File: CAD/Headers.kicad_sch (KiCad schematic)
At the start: 62 parts, among them J1 SWD, J10 OUT_0, J11 OUT_1, J12 OUT_2, J13 TEMP_0, J14 TEMP_1, J15 TEMP_2, J16 EXPANSION, J17 ESP_DB, J18 250-502/000-006, J19 A2543WV-5P, J2 A2543WV-2P, J20 IO_1, J21 IO_2, J22 A2543WV-2P, J23 CAN_1_OUT, J24 DRIVER_2, J25 DRIVER_1, J26 DRIVER_0, J28 SPI_DB, J3 OUT_6, J30 LASER/VFD, J31 IO_3, J33 A2543WV-4P, J34 A2543WV-4P, J35 DRIVER_3, J36 DRIVER_4, J37 DRIVER_5, J38 CAN_0_OUT, J39 PANELDUE_SD, J4 OUT_7, J41 TEMP_3, J42 DS_LED, J44 IO_7_ISO_OUT, J47 IO_8_ISO_OUT, J48 SBC, J49 A2543WV-2P, J5 OUT_8, J50 EXT_5V_IN, J51 IO_4, J53 IO_5, J54 IO_6, J55 IO_7, J56 IO_8, J59 A2543WV-2P, J6 OUT_3, J60 A2543WV-2P, J61 IO_7_ISO_IN, J62 IO_8_ISO_IN, J7 OUT_4, J8 OUT_5

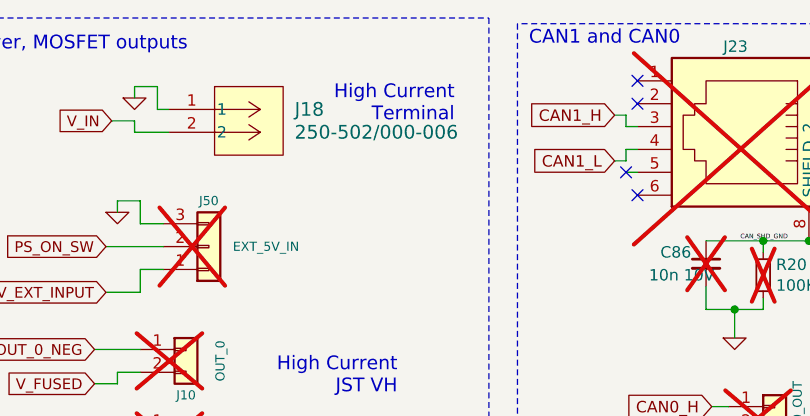
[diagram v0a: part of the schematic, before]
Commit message: Fix Part Name
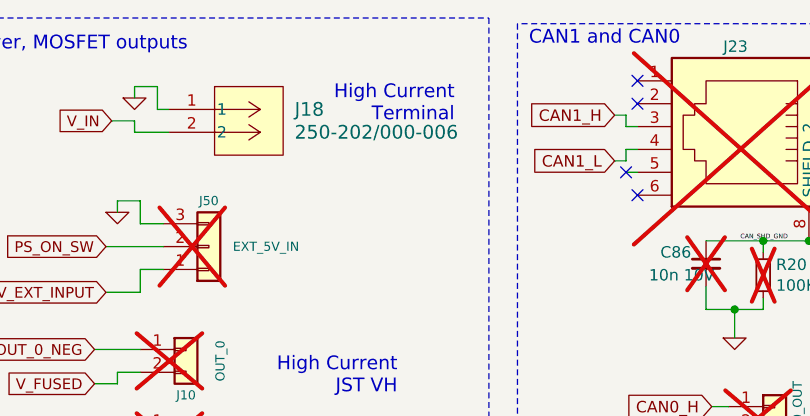
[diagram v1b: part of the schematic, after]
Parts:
- J18: value 250-502/000-006 -> 250-202/000-006; footprint 3DPotter:CONN2_250-502&slash_000-006_WAG -> 3DPotter:CONN2_250-202&slash_000-006_WAG; LCSC (none) -> C2765061
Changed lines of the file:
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@@
 			)
 		)
-		(property "Value" "250-502/000-006"
+		(property "Value" "250-202/000-006"
 			(at 53.34 26.6699 0)
 			(effects
@@
 			)
 		)
-		(property "Footprint" "3DPotter:CONN2_250-502&slash_000-006_WAG"
+		(property "Footprint" "3DPotter:CONN2_250-202&slash_000-006_WAG"
 			(at 48.006 30.226 0)
 			(effects
@@
 			)
 		)
-		(property "Datasheet" "250-502/000-006"
+		(property "Datasheet" "250-202/000-006"
 			(at 48.514 34.29 0)
 			(effects
@@
 				)
 				(hide yes)
+			)
+		)
+		(property "LCSC" "C2765061"
+			(at 39.37 24.13 0)
+			(effects
+				(font
+					(size 1.524 1.524)
+				)
+				(hide yes)

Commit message: Wago confuses me
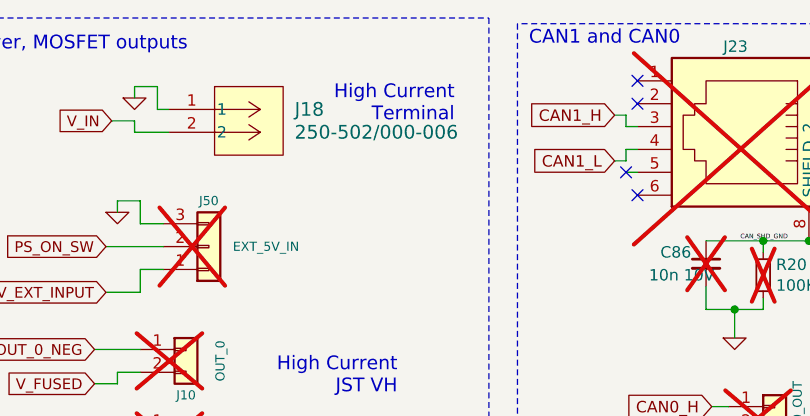
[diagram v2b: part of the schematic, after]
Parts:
- J18: value 250-202/000-006 -> 250-502/000-006; footprint 3DPotter:CONN2_250-202&slash_000-006_WAG -> 3DPotter:CONN2_250-502&slash_000-006_WAG; LCSC C2765061 -> C3309714
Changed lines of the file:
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@@
 			)
 		)
-		(property "Value" "250-202/000-006"
+		(property "Value" "250-502/000-006"
 			(at 53.34 26.6699 0)
 			(effects
@@
 			)
 		)
-		(property "Footprint" "3DPotter:CONN2_250-202&slash_000-006_WAG"
+		(property "Footprint" "3DPotter:CONN2_250-502&slash_000-006_WAG"
 			(at 48.006 30.226 0)
 			(effects
@@
 			)
 		)
-		(property "Datasheet" "250-202/000-006"
+		(property "Datasheet" "250-502/000-006"
 			(at 48.514 34.29 0)
 			(effects
@@
 			)
 		)
-		(property "LCSC" "C2765061"
+		(property "LCSC" "C3309714"
 			(at 39.37 24.13 0)
 			(effects
